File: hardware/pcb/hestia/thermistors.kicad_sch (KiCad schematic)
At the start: 56 parts, among them J12 B2B-ZR, J13 B2B-ZR, J14 B2B-ZR, J15 B2B-ZR, J16 B2B-ZR, J7 B2B-ZR, J8 B2B-ZR, U4 MAX31725MTA+T, U5 MAX31725MTA+T, U6 MAX31725MTA+T, U7 MAX31725MTA+T

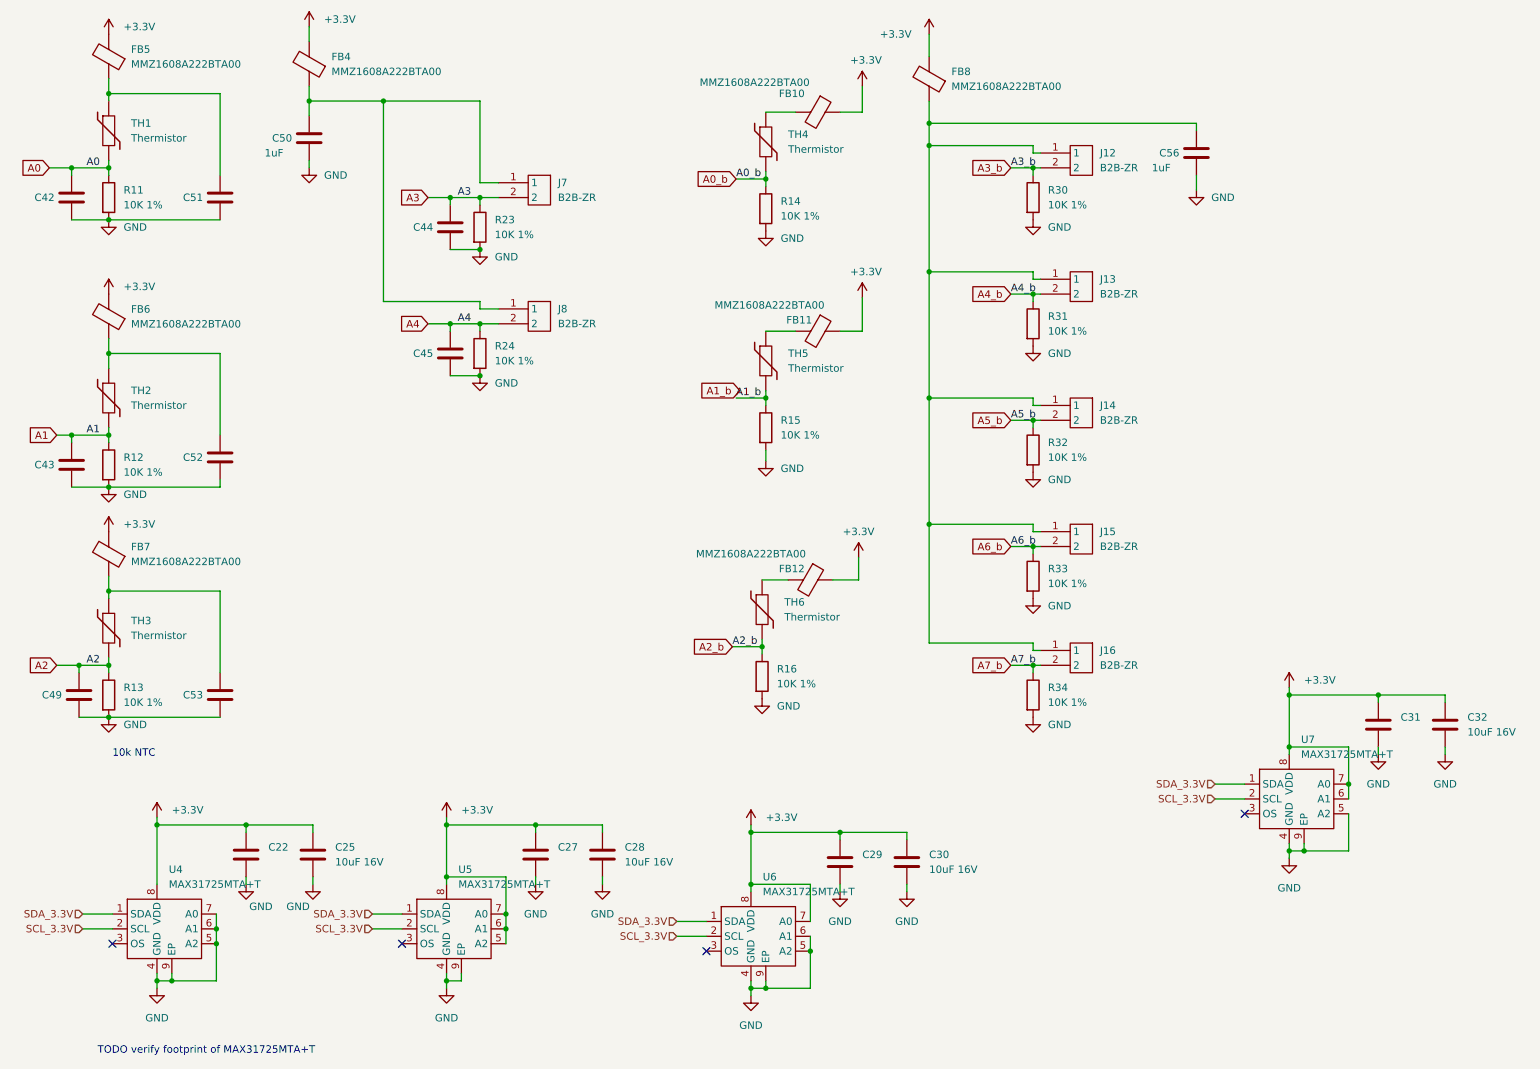
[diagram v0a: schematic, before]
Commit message: pcb: disable undervoltage latch on 3.3V regulator
- replace C3 with 0R to connect LDELAY to GND
- update footprint on PCB
- fixes #18, fixes #25
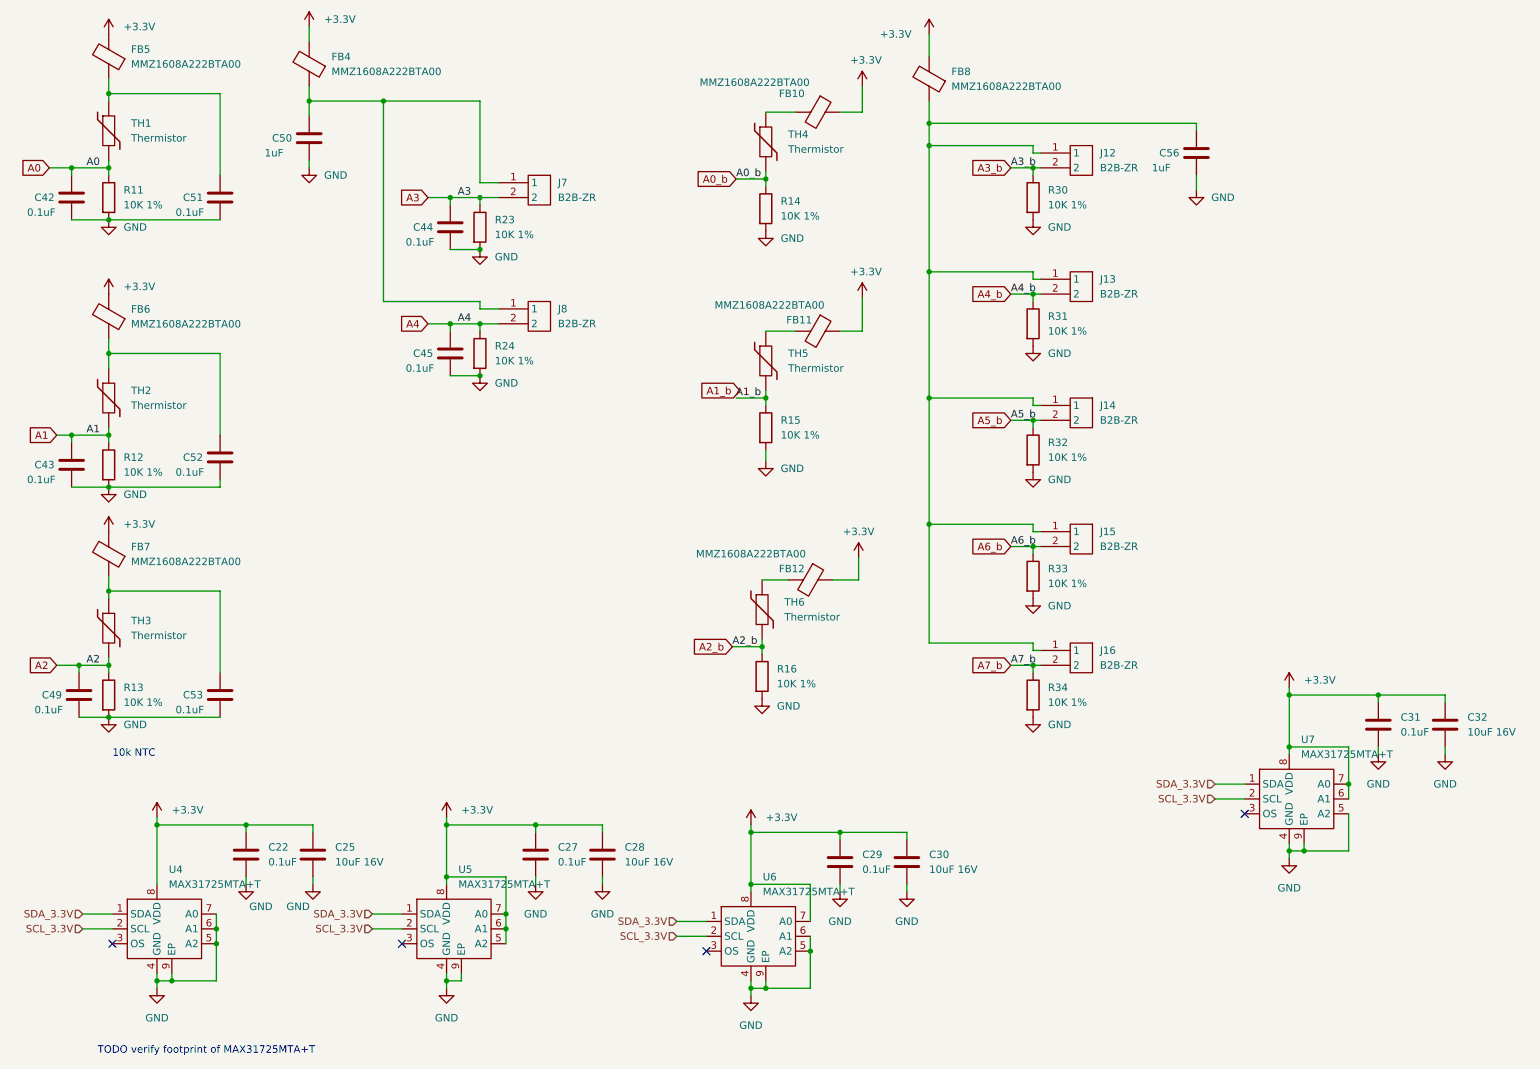
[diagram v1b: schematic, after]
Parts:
- C22, C27, C29, C31, C42, C43, C44, C45, C49, C51, C52, C53: value (none) -> 0.1uF; footprint (none) -> Capacitor_SMD:C_0603_1608Metric_Pad1.08x0.95mm_HandSolder
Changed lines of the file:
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@@
       (effects (font (size 1.27 1.27)) (justify left))
     )
-    (property "Value" "" (id 1) (at 43.815 92.71 0)
-      (effects (font (size 1.27 1.27)) (justify left))
-    )
-    (property "Footprint" "" (id 2) (at 52.4002 93.98 0)
+    (property "Value" "0.1uF" (id 1) (at 43.815 92.71 0)
+      (effects (font (size 1.27 1.27)) (justify left))
+    )
+    (property "Footprint" "Capacitor_SMD:C_0603_1608Metric_Pad1.08x0.95mm_HandSolder" (id 2) (at 52.4002 93.98 0)
       (effects (font (size 1.27 1.27)) hide)
     )
@@
       (effects (font (size 1.27 1.27)) (justify left))
     )
-    (property "Value" "" (id 1) (at 43.815 48.26 0)
-      (effects (font (size 1.27 1.27)) (justify left))
-    )
-    (property "Footprint" "" (id 2) (at 52.4002 49.53 0)
+    (property "Value" "0.1uF" (id 1) (at 43.815 48.26 0)
+      (effects (font (size 1.27 1.27)) (justify left))
+    )
+    (property "Footprint" "Capacitor_SMD:C_0603_1608Metric_Pad1.08x0.95mm_HandSolder" (id 2) (at 52.4002 49.53 0)
       (effects (font (size 1.27 1.27)) hide)
     )
@@
       (effects (font (size 1.27 1.27)) (justify left))
     )
-    (property "Value" "" (id 1) (at 43.815 133.35 0)
-      (effects (font (size 1.27 1.27)) (justify left))
-    )
-    (property "Footprint" "" (id 2) (at 52.4002 134.62 0)
+    (property "Value" "0.1uF" (id 1) (at 43.815 133.35 0)
+      (effects (font (size 1.27 1.27)) (justify left))
+    )
+    (property "Footprint" "Capacitor_SMD:C_0603_1608Metric_Pad1.08x0.95mm_HandSolder" (id 2) (at 52.4002 134.62 0)
       (effects (font (size 1.27 1.27)) hide)
     )
@@
       (effects (font (size 1.27 1.27)) (justify left))
     )
-    (property "Value" "" (id 1) (at 83.185 53.34 0)
-      (effects (font (size 1.27 1.27)) (justify left))
-    )
-    (property "Footprint" "" (id 2) (at 91.7702 54.61 0)
+    (property "Value" "0.1uF" (id 1) (at 83.185 53.34 0)
+      (effects (font (size 1.27 1.27)) (justify left))
+    )
+    (property "Footprint" "Capacitor_SMD:C_0603_1608Metric_Pad1.08x0.95mm_HandSolder" (id 2) (at 91.7702 54.61 0)
       (effects (font (size 1.27 1.27)) hide)
     )
@@
       (effects (font (size 1.27 1.27)) (justify left))
     )
-    (property "Value" "" (id 1) (at 59.69 159.3849 0)
-      (effects (font (size 1.27 1.27)) (justify left))
-    )
-    (property "Footprint" "" (id 2) (at 56.8452 161.925 0)
+    (property "Value" "0.1uF" (id 1) (at 59.69 159.3849 0)
+      (effects (font (size 1.27 1.27)) (justify left))
+    )
+    (property "Footprint" "Capacitor_SMD:C_0603_1608Metric_Pad1.08x0.95mm_HandSolder" (id 2) (at 56.8452 161.925 0)
       (effects (font (size 1.27 1.27)) hide)
     )
@@
       (effects (font (size 1.27 1.27)) (justify left))
     )
-    (property "Value" "" (id 1) (at 19.685 133.35 0)
-      (effects (font (size 1.27 1.27)) (justify left))
-    )
-    (property "Footprint" "" (id 2) (at 28.2702 134.62 0)
+    (property "Value" "0.1uF" (id 1) (at 19.685 133.35 0)
+      (effects (font (size 1.27 1.27)) (justify left))
+    )
+    (property "Footprint" "Capacitor_SMD:C_0603_1608Metric_Pad1.08x0.95mm_HandSolder" (id 2) (at 28.2702 134.62 0)
       (effects (font (size 1.27 1.27)) hide)
     )
@@
       (effects (font (size 1.27 1.27)) (justify left))
     )
-    (property "Value" "" (id 1) (at 253.365 137.1599 0)
-      (effects (font (size 1.27 1.27)) (justify left))
-    )
-    (property "Footprint" "" (id 2) (at 250.5202 139.7 0)
+    (property "Value" "0.1uF" (id 1) (at 253.365 137.1599 0)
+      (effects (font (size 1.27 1.27)) (justify left))
+    )
+    (property "Footprint" "Capacitor_SMD:C_0603_1608Metric_Pad1.08x0.95mm_HandSolder" (id 2) (at 250.5202 139.7 0)
       (effects (font (size 1.27 1.27)) hide)
     )
@@
       (effects (font (size 1.27 1.27)) (justify left))
     )
-    (property "Value" "" (id 1) (at 18.415 48.26 0)
-      (effects (font (size 1.27 1.27)) (justify left))
-    )
-    (property "Footprint" "" (id 2) (at 27.0002 49.53 0)
+    (property "Value" "0.1uF" (id 1) (at 18.415 48.26 0)
+      (effects (font (size 1.27 1.27)) (justify left))
+    )
+    (property "Footprint" "Capacitor_SMD:C_0603_1608Metric_Pad1.08x0.95mm_HandSolder" (id 2) (at 27.0002 49.53 0)
       (effects (font (size 1.27 1.27)) hide)
     )
@@
       (effects (font (size 1.27 1.27)) (justify left))
     )
-    (property "Value" "" (id 1) (at 83.185 74.93 0)
-      (effects (font (size 1.27 1.27)) (justify left))
-    )
-    (property "Footprint" "" (id 2) (at 91.7702 76.2 0)
+    (property "Value" "0.1uF" (id 1) (at 83.185 74.93 0)
+      (effects (font (size 1.27 1.27)) (justify left))
+    )
+    (property "Footprint" "Capacitor_SMD:C_0603_1608Metric_Pad1.08x0.95mm_HandSolder" (id 2) (at 91.7702 76.2 0)
       (effects (font (size 1.27 1.27)) hide)
     )
@@
       (effects (font (size 1.27 1.27)) (justify left))
     )
-    (property "Value" "" (id 1) (at 18.415 93.98 0)
-      (effects (font (size 1.27 1.27)) (justify left))
-    )
-    (property "Footprint" "" (id 2) (at 27.0002 95.25 0)
+    (property "Value" "0.1uF" (id 1) (at 18.415 93.98 0)
+      (effects (font (size 1.27 1.27)) (justify left))
+    )
+    (property "Footprint" "Capacitor_SMD:C_0603_1608Metric_Pad1.08x0.95mm_HandSolder" (id 2) (at 27.0002 95.25 0)
       (effects (font (size 1.27 1.27)) hide)
     )
@@
       (effects (font (size 1.27 1.27)) (justify left))
     )
-    (property "Value" "" (id 1) (at 109.22 159.3849 0)
-      (effects (font (size 1.27 1.27)) (justify left))
-    )
-    (property "Footprint" "" (id 2) (at 106.3752 161.925 0)
+    (property "Value" "0.1uF" (id 1) (at 109.22 159.3849 0)
+      (effects (font (size 1.27 1.27)) (justify left))
+    )
+    (property "Footprint" "Capacitor_SMD:C_0603_1608Metric_Pad1.08x0.95mm_HandSolder" (id 2) (at 106.3752 161.925 0)
       (effects (font (size 1.27 1.27)) hide)
     )
@@
       (effects (font (size 1.27 1.27)) (justify left))
     )
-    (property "Value" "" (id 1) (at 161.29 160.6549 0)
-      (effects (font (size 1.27 1.27)) (justify left))
-    )
-    (property "Footprint" "" (id 2) (at 158.4452 163.195 0)
-      (effects (font (size 1.27 1.27)) hide)
-    )
+    (property "Value" "0.1uF" (id 1) (at 161.29 160.6549 0)
+      (effects (font (size 1.27 1.27)) (justify left))
+    )
+    (property "Footprint" "Capacitor_SMD:C_0603_1608Metric_Pad1.08x0.95mm_HandSolder" (id 2) (at 158.4452 163.195 0)
+      (effects (font (size 1.27 1.27)) hide)
+    )

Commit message: change Y2 to 14.7456MHz because 7.3728MHz would have required the bigger size crystal pad. chose xtal load cap 12.5pf and 12pf for xtals. chose 20pf ext load caps to suit for C11,C12,C13,C14. Change D6 to FSV340AF - same family just 40V reverse voltage max rather than 30V reverse voltage max because FSV330AF was out of stock. Added some more digikey part numbers
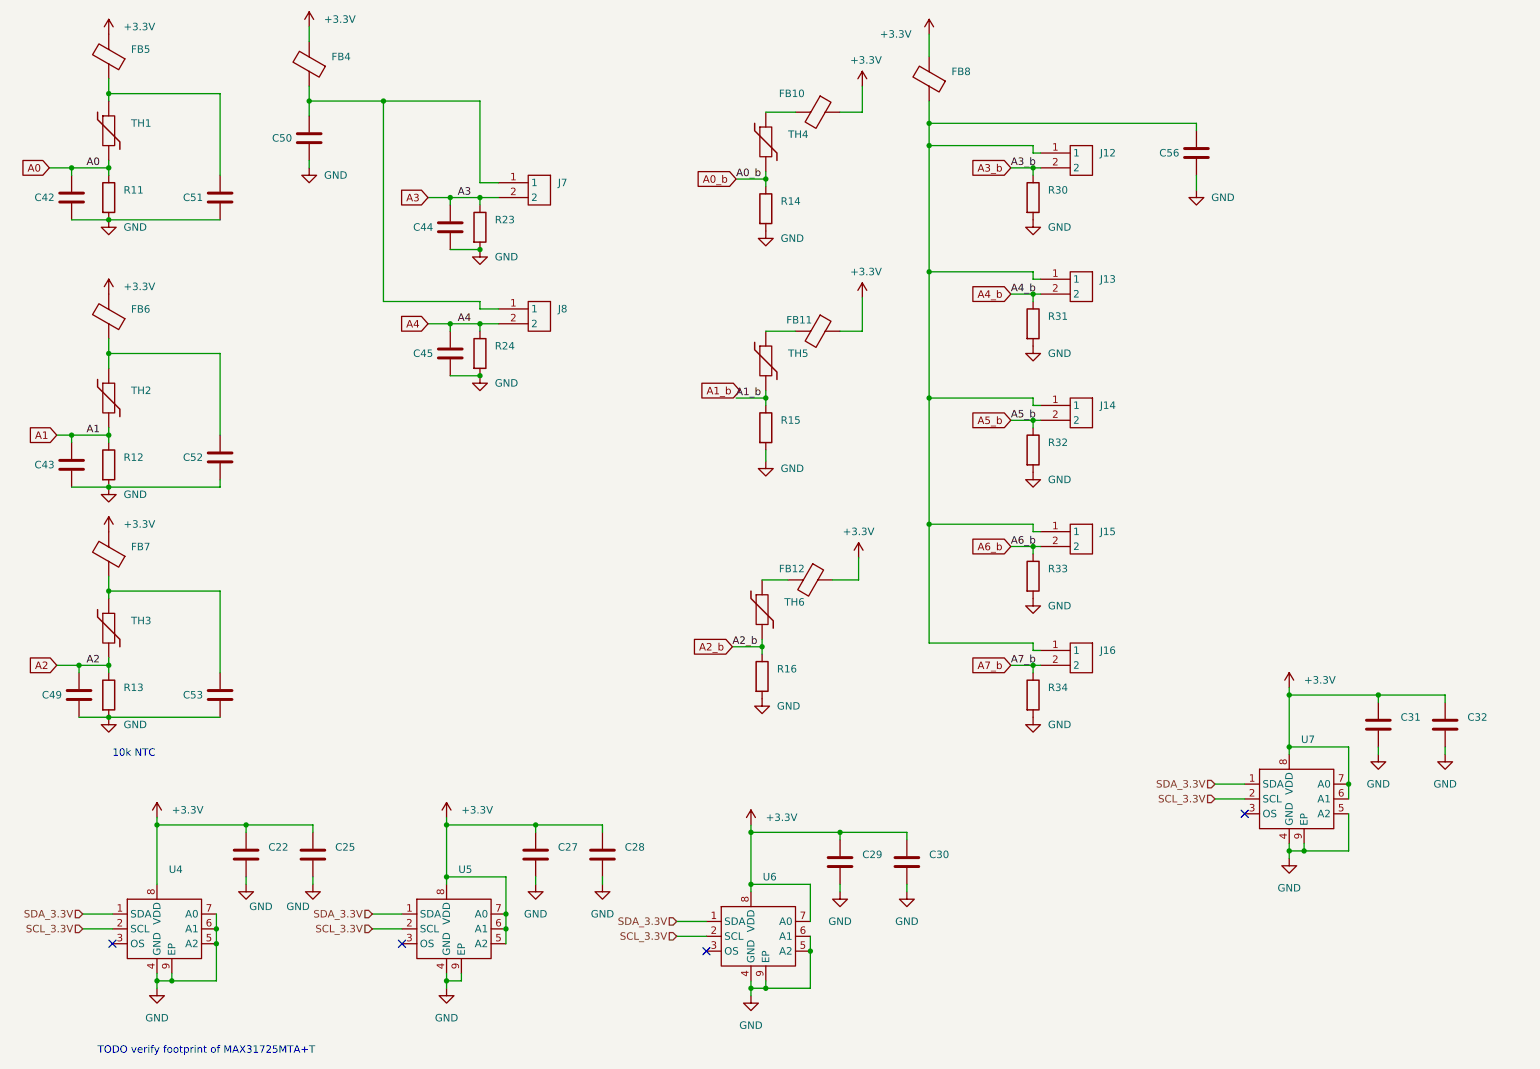
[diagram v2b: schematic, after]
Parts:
- C22, C27, C29, C31, C42, C43, C44, C45, C49, C51, C52, C53: value 0.1uF -> (none); footprint Capacitor_SMD:C_0603_1608Metric_Pad1.08x0.95mm_HandSolder -> (none)
- C25, C28, C30, C32: value 10uF 16V -> (none); footprint Capacitor_SMD:C_0603_1608Metric_Pad1.08x0.95mm_HandSolder -> (none)
- C50, C56: value 1uF -> (none); footprint Capacitor_SMD:C_0603_1608Metric_Pad1.08x0.95mm_HandSolder -> (none)
- FB10, FB11, FB12, FB4, FB5, FB6, FB7, FB8: value MMZ1608A222BTA00 -> (none); footprint Resistor_SMD:R_0603_1608Metric_Pad0.98x0.95mm_HandSolder -> (none)
- J12, J13, J14, J15, J16, J7, J8: value B2B-ZR -> (none); footprint Hestia:B2B-ZR(LF)(SN) -> (none)
- R11, R12, R13, R14, R15, R16, R23, R24, R30, R31, R32, R33, R34: value 10K 1% -> (none); footprint Resistor_SMD:R_0603_1608Metric_Pad0.98x0.95mm_HandSolder -> (none)
- TH1, TH2, TH3, TH4, TH5, TH6: value Thermistor -> (none); footprint Resistor_SMD:R_0603_1608Metric_Pad0.98x0.95mm_HandSolder -> (none)
- U4, U5, U6, U7: value MAX31725MTA+T -> (none); footprint Package_DFN_QFN:DFN-8-1EP_3x3mm_P0.65mm_EP1.55x2.4mm -> (none)

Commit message: Restore lost footprints in schematics
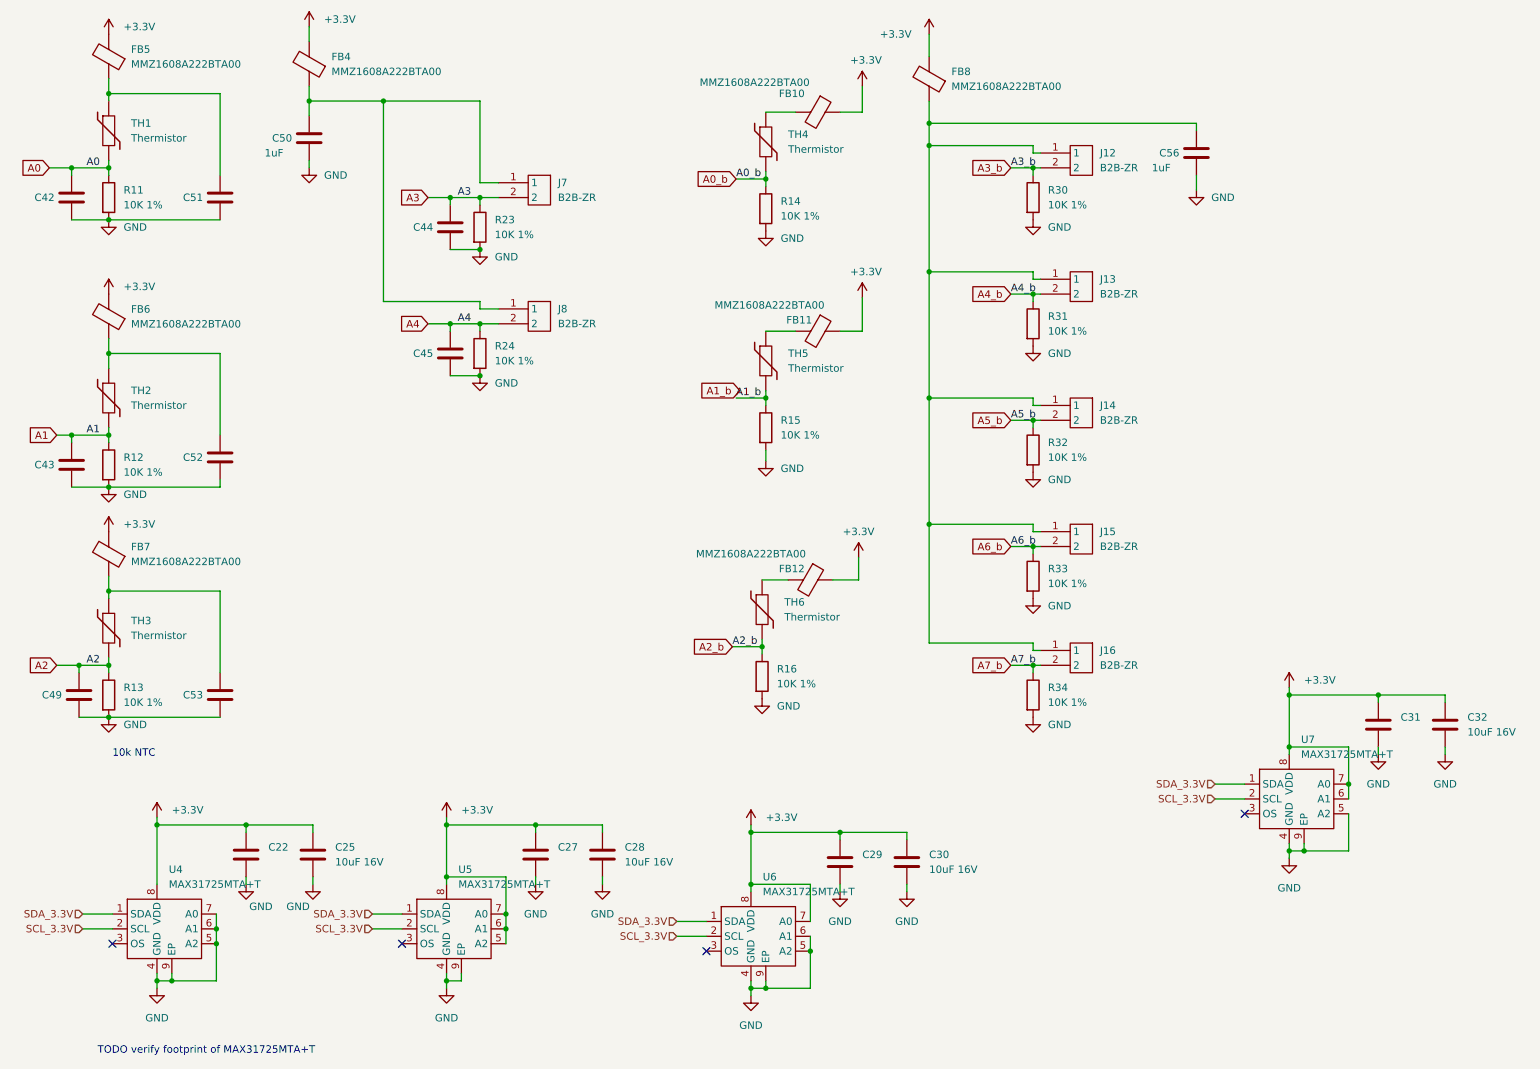
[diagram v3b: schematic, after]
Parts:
- C25, C28, C30, C32: value (none) -> 10uF 16V; footprint (none) -> Capacitor_SMD:C_0603_1608Metric_Pad1.08x0.95mm_HandSolder
- C50, C56: value (none) -> 1uF; footprint (none) -> Capacitor_SMD:C_0603_1608Metric_Pad1.08x0.95mm_HandSolder
- FB10, FB11, FB12, FB4, FB5, FB6, FB7, FB8: value (none) -> MMZ1608A222BTA00; footprint (none) -> Resistor_SMD:R_0603_1608Metric_Pad0.98x0.95mm_HandSolder
- J12, J13, J14, J15, J16, J7, J8: value (none) -> B2B-ZR; footprint (none) -> Hestia:B2B-ZR(LF)(SN)
- R11, R12, R13, R14, R15, R16, R23, R24, R30, R31, R32, R33, R34: value (none) -> 10K 1%; footprint (none) -> Resistor_SMD:R_0603_1608Metric_Pad0.98x0.95mm_HandSolder
- TH1, TH2, TH3, TH4, TH5, TH6: value (none) -> Thermistor; footprint (none) -> Resistor_SMD:R_0603_1608Metric_Pad0.98x0.95mm_HandSolder
- U4, U5, U6, U7: value (none) -> MAX31725MTA+T; footprint (none) -> Package_DFN_QFN:DFN-8-1EP_3x3mm_P0.65mm_EP1.55x2.4mm
